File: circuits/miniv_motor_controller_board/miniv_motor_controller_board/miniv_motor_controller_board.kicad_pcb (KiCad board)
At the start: 2 copper layers, 78 x 102 mm, 4 parts

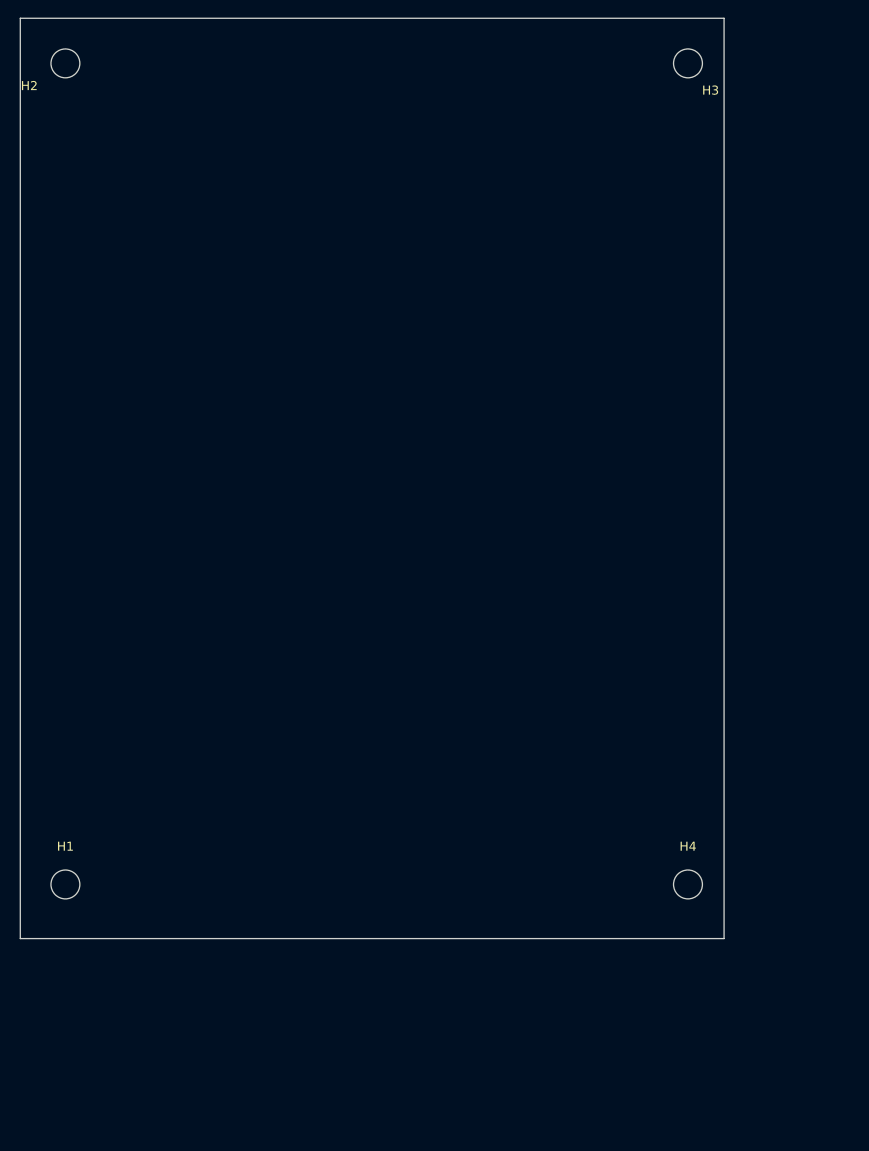
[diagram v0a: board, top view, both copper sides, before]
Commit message: update board
Signed-off-by: Masaya Kataoka <ms.kataoka@gmail.com>
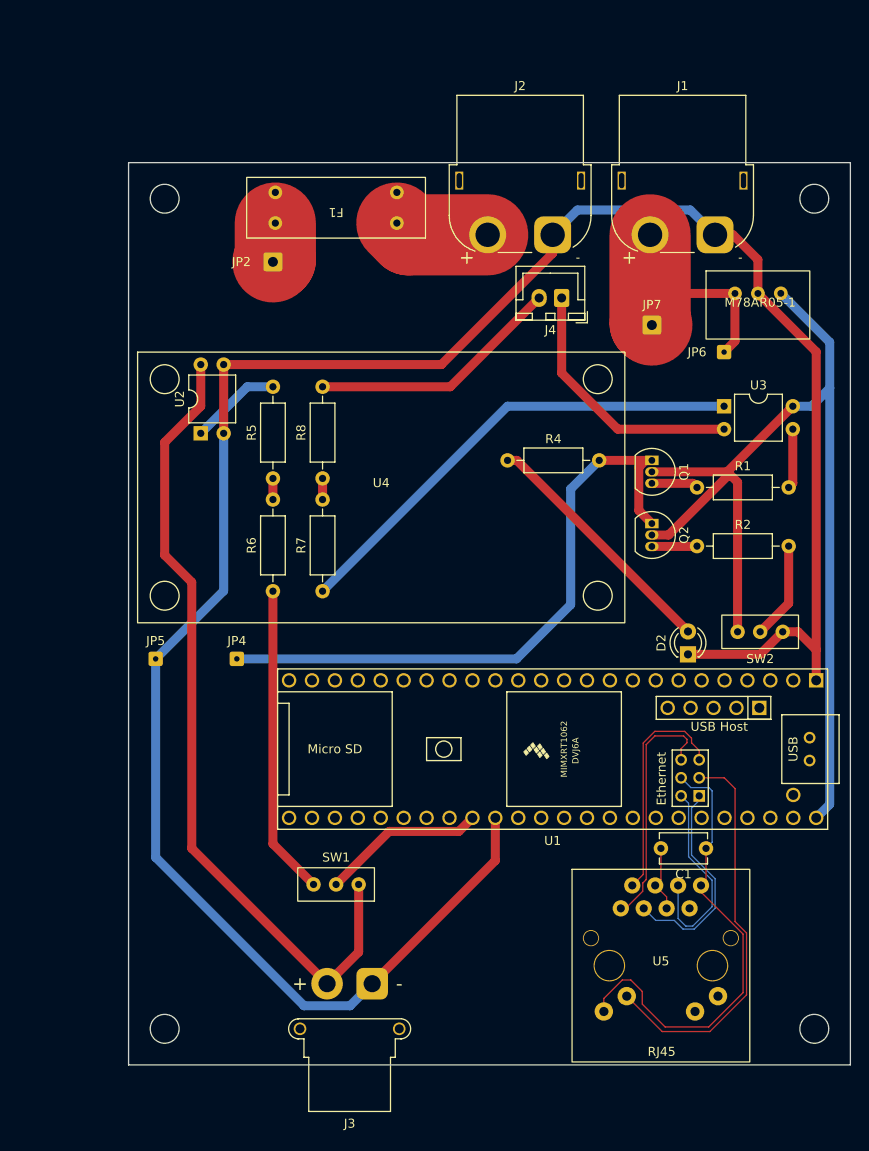
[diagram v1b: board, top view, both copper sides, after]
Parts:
- added C1: 0.1u, Capacitor_THT:C_Disc_D5.1mm_W3.2mm_P5.00mm, F.Cu at (106.0, 126.0)
- added D2: LED, LED_THT:LED_D3.0mm, F.Cu at (104.0, 104.5)
- added F1: Fuse, 3557-15:3557-15, F.Cu at (65.0, 55.0)
- added J1: DC_in, Connector_AMASS:AMASS_XT60PW-F_1x02_P7.20mm_Horizontal, F.Cu at (107.0, 58.0)
- added J2: T200_ESC_power, Connector_AMASS:AMASS_XT60PW-F_1x02_P7.20mm_Horizontal, F.Cu at (89.0, 58.0)
- added J3: T200_ESC_signal, Connector_AMASS:AMASS_XT30PW-F_1x02_P2.50mm_Horizontal, F.Cu at (69.0, 141.0)
- added J4: Conn_EStop_Signal, Connector_JST:JST_XH_B2B-XH-A_1x02_P2.50mm_Vertical, F.Cu at (90.0, 65.0)
- added JP2: Relay_NO, Connector_Wire:SolderWire-0.5sqmm_1x01_D0.9mm_OD2.1mm, F.Cu at (58.0, 61.0)
- added JP4: Relay_SIG, Connector_Wire:SolderWire-0.1sqmm_1x01_D0.4mm_OD1mm, F.Cu at (54.0, 105.0)
- added JP5: Relay_GND, Connector_Wire:SolderWire-0.1sqmm_1x01_D0.4mm_OD1mm, F.Cu at (45.0, 105.0)
- added JP6: Relay_VCC, Connector_Wire:SolderWire-0.1sqmm_1x01_D0.4mm_OD1mm, F.Cu at (108.0, 71.0)
- added JP7: Relay_COM, Connector_Wire:SolderWire-0.5sqmm_1x01_D0.9mm_OD2.1mm, F.Cu at (100.0, 68.0)
- added M78AR05-1: ~, M78AR05-1:M78AR05-1, F.Cu at (112.0, 66.0)
- added Q1: 2SC1815, Package_TO_SOT_THT:TO-92_Inline, F.Cu at (100.0, 83.0)
- added Q2: 2SC1815, Package_TO_SOT_THT:TO-92_Inline, F.Cu at (100.0, 90.0)
- added R1: 100k, Resistor_THT:R_Axial_DIN0207_L6.3mm_D2.5mm_P10.16mm_Horizontal, F.Cu at (105.0, 86.0)
- added R2: 100k, Resistor_THT:R_Axial_DIN0207_L6.3mm_D2.5mm_P10.16mm_Horizontal, F.Cu at (105.0, 92.5)
- added R4: 470, Resistor_THT:R_Axial_DIN0207_L6.3mm_D2.5mm_P10.16mm_Horizontal, F.Cu at (84.0, 83.0)
- added R5: 390, Resistor_THT:R_Axial_DIN0207_L6.3mm_D2.5mm_P10.16mm_Horizontal, F.Cu at (58.0, 85.0)
- added R6: 1K, Resistor_THT:R_Axial_DIN0207_L6.3mm_D2.5mm_P10.16mm_Horizontal, F.Cu at (58.0, 97.5)
- added R7: 1K, Resistor_THT:R_Axial_DIN0207_L6.3mm_D2.5mm_P10.16mm_Horizontal, F.Cu at (63.5, 97.5)
- added R8: 390, Resistor_THT:R_Axial_DIN0207_L6.3mm_D2.5mm_P10.16mm_Horizontal, F.Cu at (63.5, 85.0)
- added SW1: SW_isolation, SS-12D00G3:SS-12D00G3, F.Cu at (65.0, 130.0)
- added SW2: SW_disable_EStop, SS-12D00G3:SS-12D00G3, F.Cu at (112.0, 102.0)
- added U1: Teensy4.1, Teensy_Custom:Teensy41, F.Cu at (89.0, 115.0)
- added U2: TLP624, Package_DIP:DIP-4_W7.62mm, F.Cu at (50.0, 80.0)
- added U3: TLP624, Package_DIP:DIP-4_W7.62mm, F.Cu at (108.0, 77.0)
- added U4: ~, AE-RELAY953B-12V:AE-RELAY953B-12V, F.Cu at (70.0, 86.0)
- added U5: ~, RJLD-260YC1:RJLD-260YC1, F.Cu at (101.0, 139.0)
- moved H4 21.3 mm to (118.0, 146.0)
- moved H3 20.5 mm to (118.0, 54.0)
- moved H1 19.4 mm to (46.0, 146.0)
- moved H2 18.6 mm to (46.0, 54.0)
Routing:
- net GND: track 0.00 -> 248.8 mm
- net Net-(M78AR05-1-Vout): track 0.00 -> 114.3 mm
- net Net-(J3-Pin_2): track 0.00 -> 90.2 mm
- net Net-(JP4-A): track 0.00 -> 71.2 mm
- net Net-(R7-Pad1): track 0.00 -> 53.0 mm
- net Net-(U5-GND): track 0.00 -> 51.1 mm
- net Net-(U1-LED): track 0.00 -> 44.4 mm
- net Net-(SW1-C): track 0.00 -> 34.4 mm
- net Net-(J4-Pin_1): track 0.00 -> 28.9 mm
- net Net-(J4-Pin_2): track 0.00 -> 28.1 mm
- net Net-(D2-A): track 0.00 -> 27.9 mm
- net +12V: track 0.00 -> 27.7 mm
- net Net-(U1-T+): track 0.00 -> 27.2 mm
- net Net-(U1-T-): track 0.00 -> 25.2 mm
- net Net-(U1-R+): track 0.00 -> 23.7 mm
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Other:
- board size 78 x 102 mm -> 80 x 100 mm
